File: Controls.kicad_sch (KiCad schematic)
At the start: 10 parts, among them J1 FOOTSWITCH, J2 PCIE_FX, SW1 SW_SPDT, SW2 SW_SPDT, SW3 SW_SPDT, X1 PEDAL_COMBO_TOP

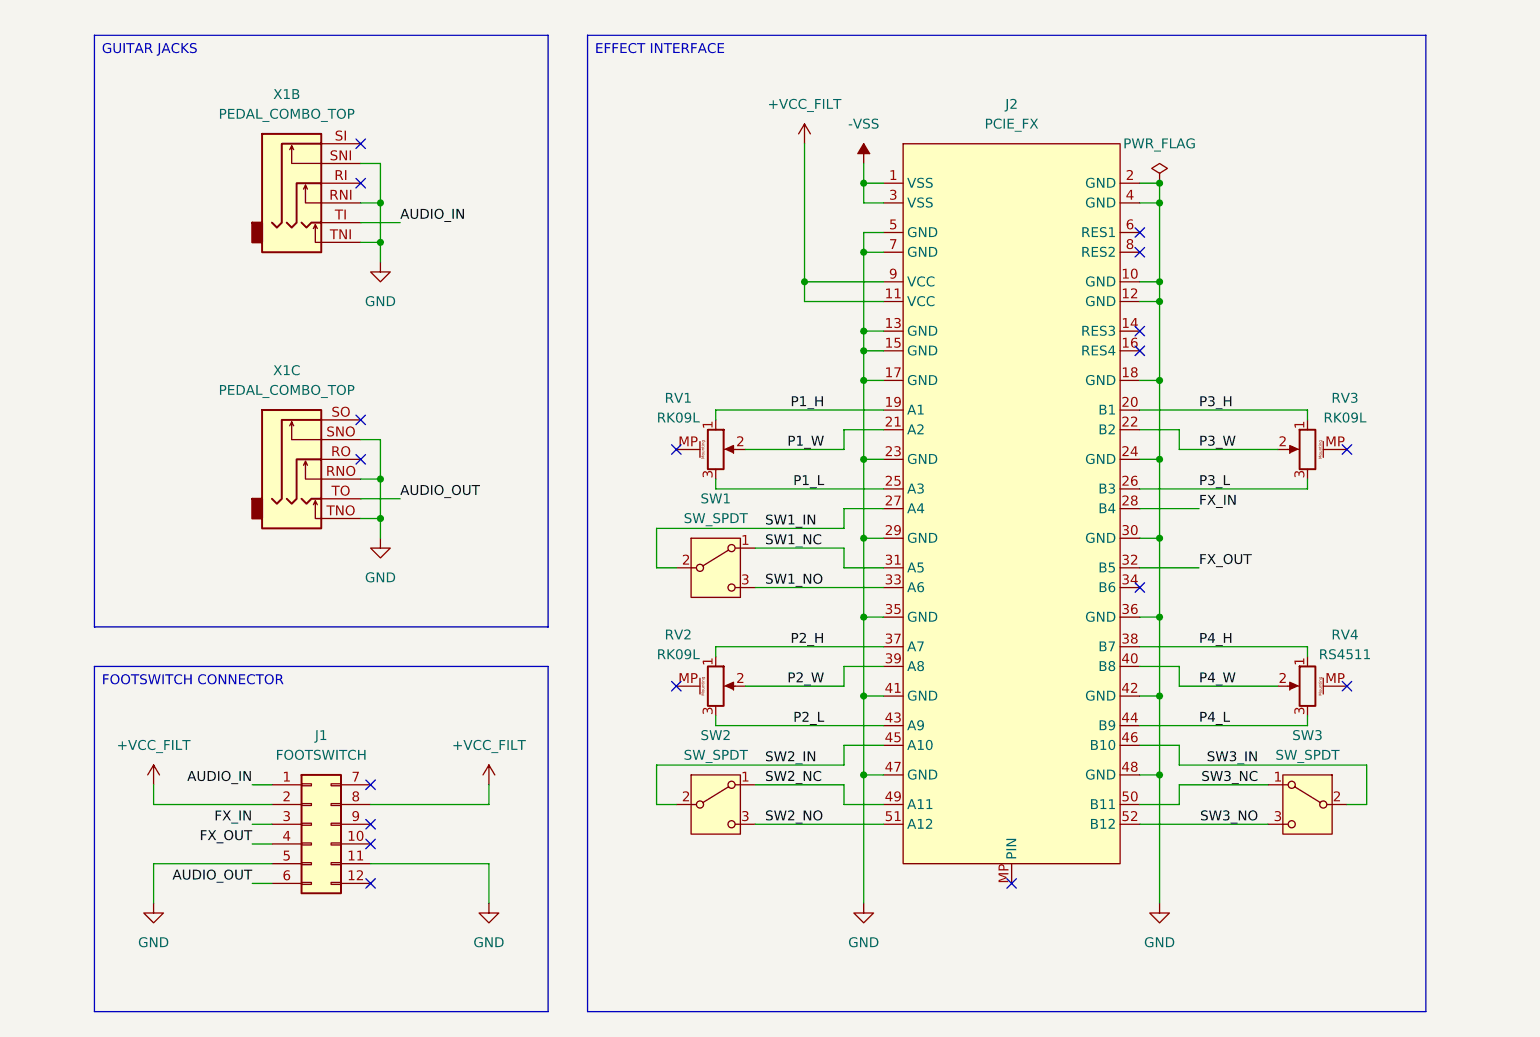
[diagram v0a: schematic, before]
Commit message: Initial layout
Finished the initial PCB layout.
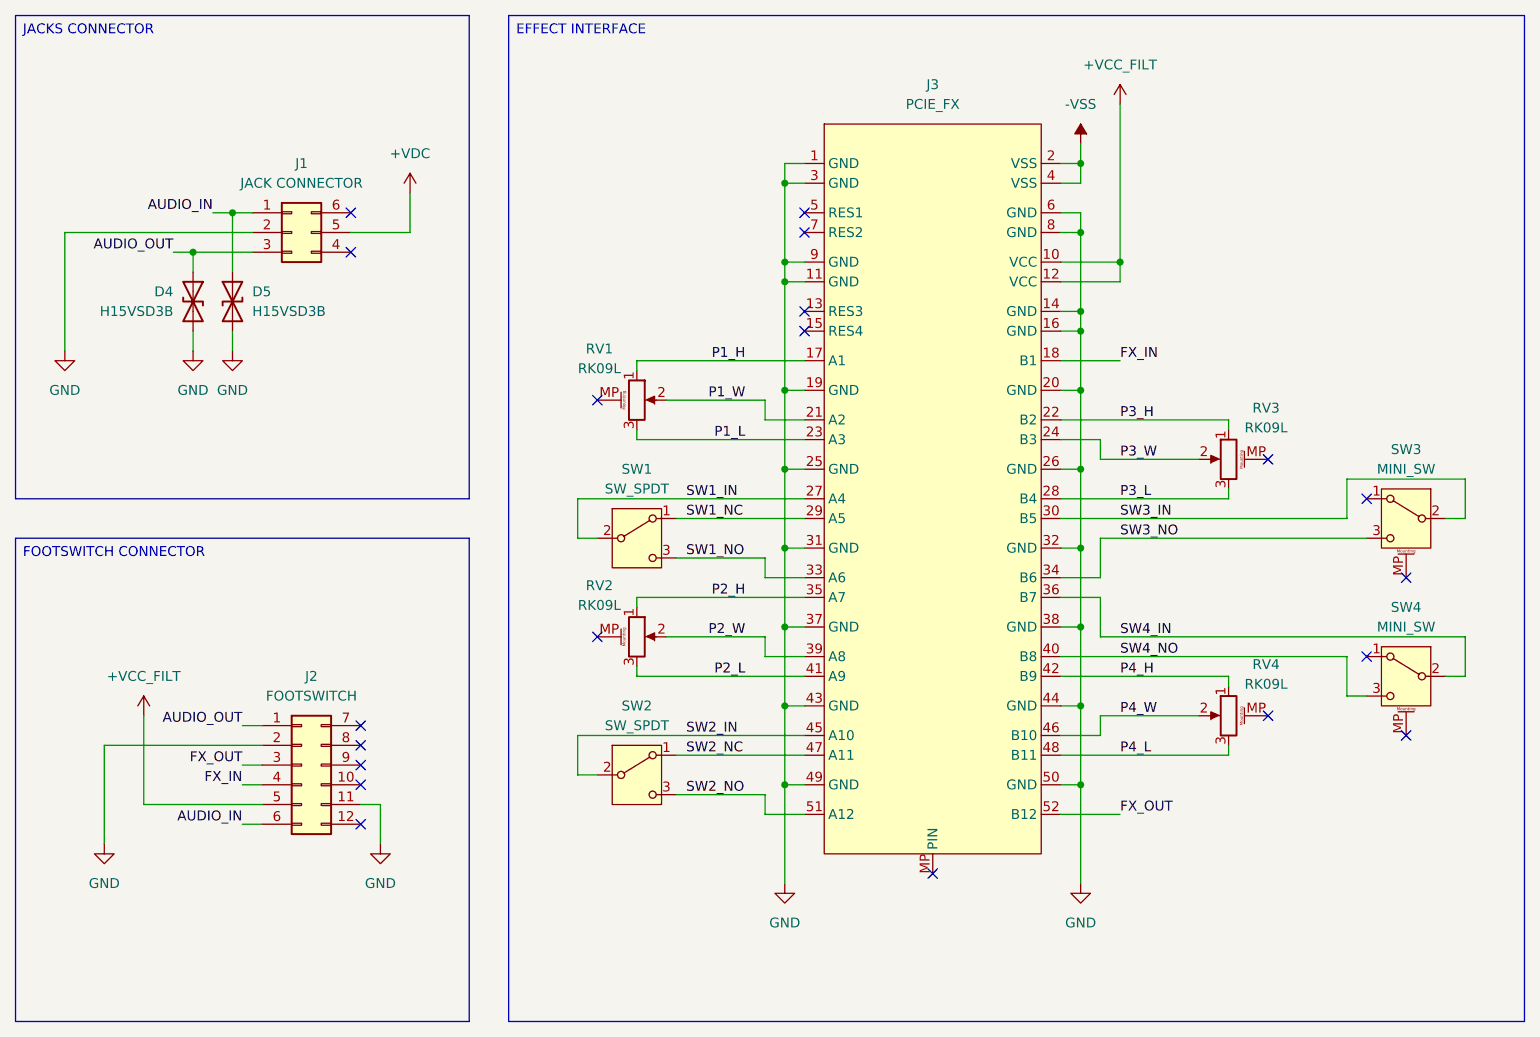
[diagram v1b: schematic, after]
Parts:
- removed SW3: SW_SPDT, Custom_Parts:SW_SPDT, symbol Switch:SW_SPDT
- removed X1: PEDAL_COMBO_TOP, Custom_Parts:PEDAL_COMBO_TOP, symbol Custom_Parts:PEDAL_COMBO_TOP
- added D4, D5: H15VSD3B, Diode_SMD:D_SOD-323, symbol Device:D_TVS
- added J1: JACK CONNECTOR, Custom_Parts:HEADER_THROUGH_2x03_P2.54mm, symbol Connector_Generic:Conn_02x03_Counter_Clockwise
- added SW3, SW4: MINI_SW, Custom_Parts:MINI_TOGGLE_SHIELD, symbol Custom_Parts:SW_SPDT_MountingPin
- RV4: value RS4511 -> RK09L; footprint Custom_Parts:RS45111A900F -> Custom_Parts:POT_SINGLE_VERTICAL_6X15
- renumbered J1 to J2, J2 to J3
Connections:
- net SW3_NC is gone; now on net GND: J3.50 (GND)
- net +VCC_FILT: now also J2.5 (Pin_5), J3.10 (VCC), J3.12 (VCC); no longer J2.2 (Pin_2), J2.8 (Pin_8), J3.11 (VCC), J3.9 (VCC)
- net -VSS: now also J3.2 (VSS), J3.4 (VSS); no longer J3.1 (VSS), J3.3 (VSS)
- net AUDIO_IN: now also J2.6 (Pin_6), D5.1 (A1), J1.1 (Pin_1); no longer J2.1 (Pin_1)
- net AUDIO_OUT: now also J2.1 (Pin_1), D4.1 (A1), J1.3 (Pin_3); no longer J2.6 (Pin_6)
- net FX_IN: now also J2.4 (Pin_4), J3.18 (B1); no longer J2.3 (Pin_3), J3.28 (B4)
- net FX_OUT: now also J2.3 (Pin_3), J3.52 (B12); no longer J2.4 (Pin_4), J3.32 (B5)
- net GND: now also J2.2 (Pin_2), J3.1 (GND), J3.11 (GND), J3.14 (GND), J3.16 (GND), J3.19 (GND), J3.20 (GND), J3.25 (GND), J3.26 (GND), J3.3 (GND), J3.31 (GND), J3.32 (GND), J3.37 (GND), J3.38 (GND), J3.43 (GND), J3.44 (GND), J3.49 (GND), J3.6 (GND), J3.8 (GND), J3.9 (GND), D4.2 (A2), D5.2 (A2), J1.2 (Pin_2); no longer J2.5 (Pin_5), J3.10 (GND), J3.12 (GND), J3.13 (GND), J3.15 (GND), J3.17 (GND), J3.18 (GND), J3.2 (GND), J3.23 (GND), J3.24 (GND), J3.29 (GND), J3.30 (GND), J3.35 (GND), J3.36 (GND), J3.4 (GND), J3.41 (GND), J3.42 (GND), J3.47 (GND), J3.48 (GND), J3.5 (GND), J3.7 (GND)
- net P1_H: now also J3.17 (A1); no longer J3.19 (A1)
- net P1_L: now also J3.23 (A3); no longer J3.25 (A3)
- net P2_H: now also J3.35 (A7); no longer J3.37 (A7)
- net P2_L: now also J3.41 (A9); no longer J3.43 (A9)
- net P3_H: now also J3.22 (B2); no longer J3.20 (B1)
- net P3_L: now also J3.28 (B4); no longer J3.26 (B3)
- net P3_W: now also J3.24 (B3); no longer J3.22 (B2)
- net P4_H: now also J3.42 (B9); no longer J3.38 (B7)
- net P4_L: now also J3.48 (B11); no longer J3.44 (B9)
- net P4_W: now also J3.46 (B10); no longer J3.40 (B8)
- net SW1_NC: now also J3.29 (A5); no longer J3.31 (A5)
- net SW2_NC: now also J3.47 (A11); no longer J3.49 (A11)
- net SW3_IN: now also J3.30 (B5), SW3.2 (B); no longer J3.46 (B10)
- net SW3_NO: now also J3.34 (B6), SW3.3 (C); no longer J3.52 (B12)
- new net +VDC: J1.5 (Pin_5)
- new net SW4_IN: J3.36 (B7), SW4.2 (B)
- new net SW4_NO: J3.40 (B8), SW4.3 (C)
- no-connect marks 18 -> 20
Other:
- moved on the sheet: J2, J3
